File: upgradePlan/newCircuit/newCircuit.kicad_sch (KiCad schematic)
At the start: 40 parts

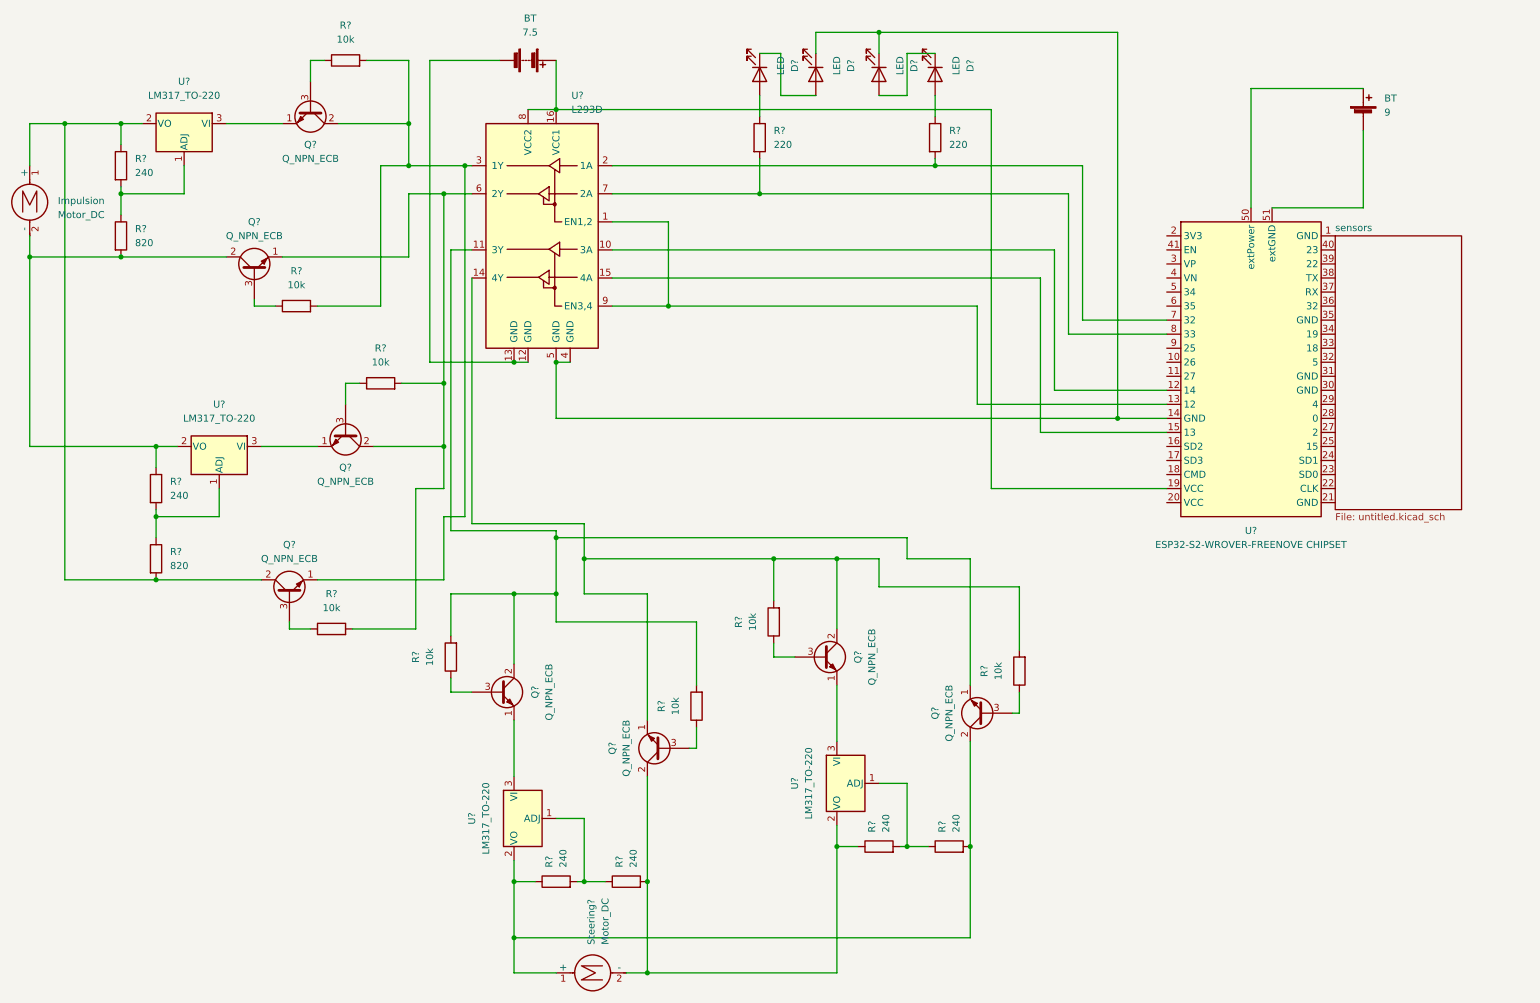
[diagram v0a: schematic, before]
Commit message: circuit V0.1
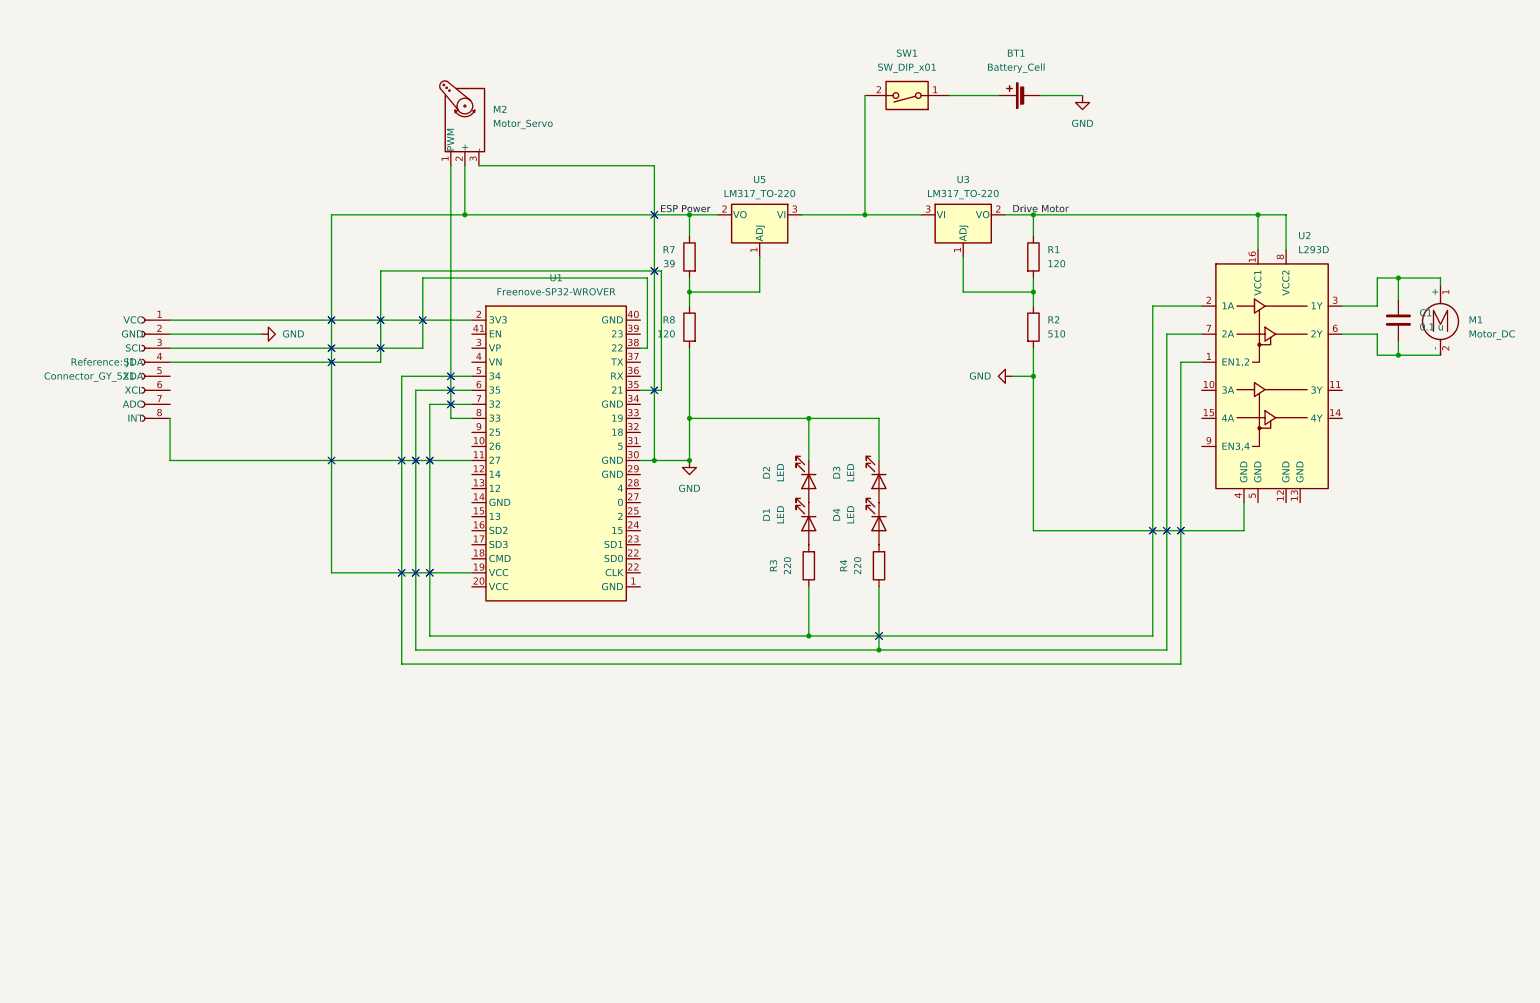
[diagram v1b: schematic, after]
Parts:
- removed BT: 9, symbol Device:Battery_Cell
- removed BT: 7.5, symbol Device:Battery
- removed D? (x4): LED, symbol Device:LED
- removed Impulsion, Steering?: Motor_DC, symbol Motor:Motor_DC
- removed Q? (x8): Q_NPN_ECB, symbol Device:Q_NPN_ECB
- removed R? (x8): 10k, symbol Device:R
- removed R? (x6): 240, symbol Device:R
- removed R? (x2): 220, symbol Device:R
- removed R? (x2): 820, symbol Device:R
- removed U? (x4): LM317_TO-220, Package_TO_SOT_THT:TO-220-3_Vertical, symbol Regulator_Linear:LM317_TO-220
- removed U?: L293D, Package_DIP:DIP-16_W7.62mm, symbol Driver_Motor:L293D
- removed U?: ESP32-S2-WROVER-FREENOVE CHIPSET, RF_Module:ESP32-S2-WROVER, symbol My_RC_Car:ESP32-S2-WROVER-FREENOVE CHIPSET
- added BT1: Battery_Cell, symbol Device:Battery_Cell
- added C1: 0.1 u, symbol Device:C
- added D1, D2, D3, D4: LED, symbol Device:LED
- added J1: Connector_GY_521, symbol Connector:Connector_GY-521
- added M1: Motor_DC, symbol Motor:Motor_DC
- added M2: Motor_Servo, symbol Motor:Motor_Servo
- added R1, R8: 120, symbol Device:R
- added R2: 510, symbol Device:R
- added R3, R4: 220, symbol Device:R
- added R7: 39, symbol Device:R
- added SW1: SW_DIP_x01, symbol Switch:SW_DIP_x01
- added U1: Freenove-SP32-WROVER, RF_Module:Freenove-ESP32-WROVER, symbol RF_Module:ESP32-S2-WROVER
- added U2: L293D, Package_DIP:DIP-16_W7.62mm, symbol Driver_Motor:L293D
- added U3, U5: LM317_TO-220, Package_TO_SOT_THT:TO-220-3_Vertical, symbol Regulator_Linear:LM317_TO-220
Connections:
- new net: C1.1, M1.1 (+), U2.3 (1Y)
- new net: C1.2, M1.2 (-), U2.6 (2Y)
- new net: M2.1 (PWM), U1.8 (33)
- new net: BT1.1 (+), SW1.1
- new net: SW1.2, U3.3 (VI), U5.3 (VI)
- new net: R1.2, R2.1, U3.1 (ADJ)
- new net: D3.2 (A), D4.1 (K)
- new net: D1.1 (K), D2.2 (A)
- new net: D1.2 (A), R3.2
- new net: J1.1 (VCC), U1.2 (3V3)
- new net: J1.3 (SCL), U1.38 (22)
- new net: J1.4 (SDA), U1.35 (21)
- new net: J1.8 (INT), U1.11 (27)
- new net: D4.2 (A), R4.2
- new net: R4.1, U1.6 (35), U2.7 (2A)
- new net: R7.2, R8.1, U5.1 (ADJ)
- new net: U1.5 (34), U2.1 (EN1,2)
- new net: R3.1, U1.7 (32), U2.2 (1A)
- new net Drive Motor: R1.1, U2.16 (VCC1), U2.8 (VCC2), U3.2 (VO)
- new net ESP Power: M2.2 (+), R7.1, U1.19 (VCC), U5.2 (VO)
- new net GND: BT1.2 (-), D2.1 (K), D3.1 (K), J1.2 (GND), M2.3 (-), R2.2, R8.2, U1.30 (GND), U2.4 (GND)
- no-connect marks 0 -> 23
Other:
- removed sheet sensors
- title: new ciruit rospCar -> (none)
